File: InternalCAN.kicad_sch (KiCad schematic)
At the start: 5 parts, among them U4 ISO1044BD, U5 CDSOT23-T24CAN

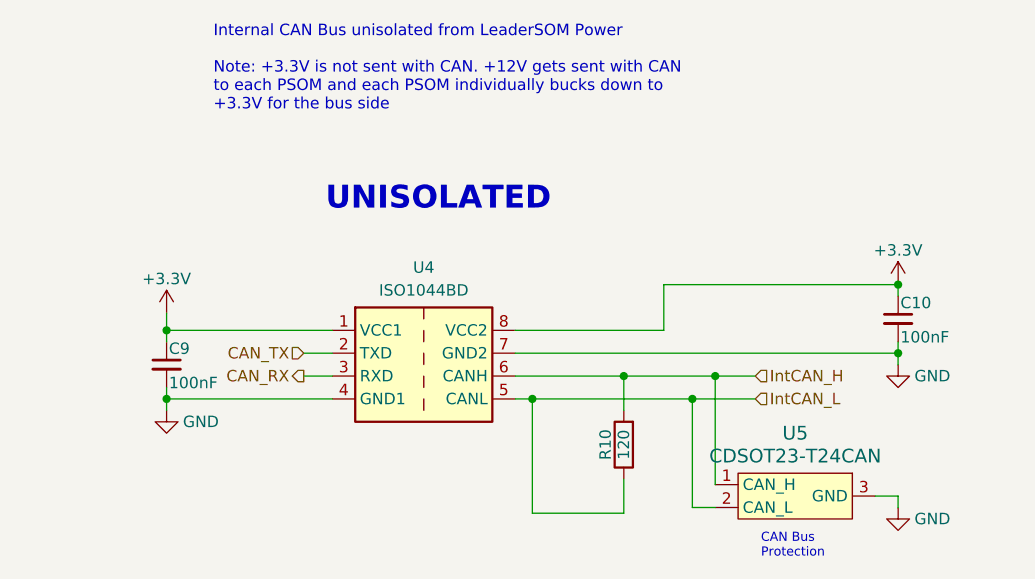
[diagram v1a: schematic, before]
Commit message: laid things out but still need to fix things :(
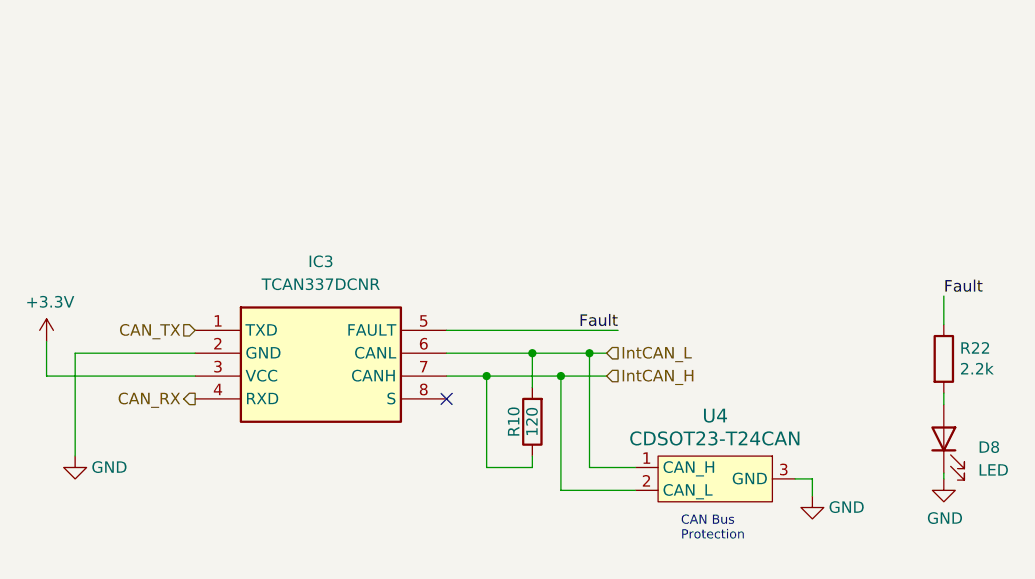
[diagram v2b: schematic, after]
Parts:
- removed C10, C9: 100nF, Capacitor_SMD:C_0805_2012Metric, symbol Device:C_Small
- removed U4: ISO1044BD, Package_SO:SSOP-8_3.9x5.05mm_P1.27mm, symbol utsvt-chips:ISO1044BD
- removed U5: CDSOT23-T24CAN, Package_TO_SOT_SMD:SOT-23W, symbol utsvt-chips:CDSOT23-T24CAN
- added D8: LED, LED_SMD:LED_0805_2012Metric, symbol Device:LED
- added IC3: TCAN337DCNR, UTSVT_ICs:SOT65P280X145-8N, symbol utsvt-chips:TCAN337DCNR
- added R22: 2.2k, Resistor_SMD:R_0805_2012Metric, symbol Device:R
- added U4: CDSOT23-T24CAN, Package_TO_SOT_SMD:SOT-23W, symbol utsvt-chips:CDSOT23-T24CAN
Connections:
- net +3.3V: now also IC3.3 (VCC)
- net CAN_RX: now also IC3.4 (RXD)
- net CAN_TX: now also IC3.1 (TXD)
- net GND: now also D8.1 (K), IC3.2 (GND), U4.3 (GND)
- net IntCAN_H: now also R10.1, IC3.7 (CANH), U4.2 (CAN_L); no longer R10.2
- net IntCAN_L: now also R10.2, IC3.6 (CANL), U4.1 (CAN_H); no longer R10.1
- new net: D8.2 (A), R22.2
- new net Fault: IC3.5 (FAULT), R22.1
- no-connect marks 0 -> 1
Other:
- note removed: "Internal CAN Bus unisolated from LeaderSOM Power"
- note removed: "Note: +3.3V is not sent with CAN. +12V gets sent with CAN to each PSOM and each PSOM individually bucks down to +3.3V for the bus side"
- note removed: "UNISOLATED"
